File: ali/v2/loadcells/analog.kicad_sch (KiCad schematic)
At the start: 57 parts, among them J10 Conn_01x04, J11 Conn_01x04, J12 Conn_01x04, J13 Conn_01x04, J14 Conn_01x04, J9 Conn_01x04, U5 ADS124S08

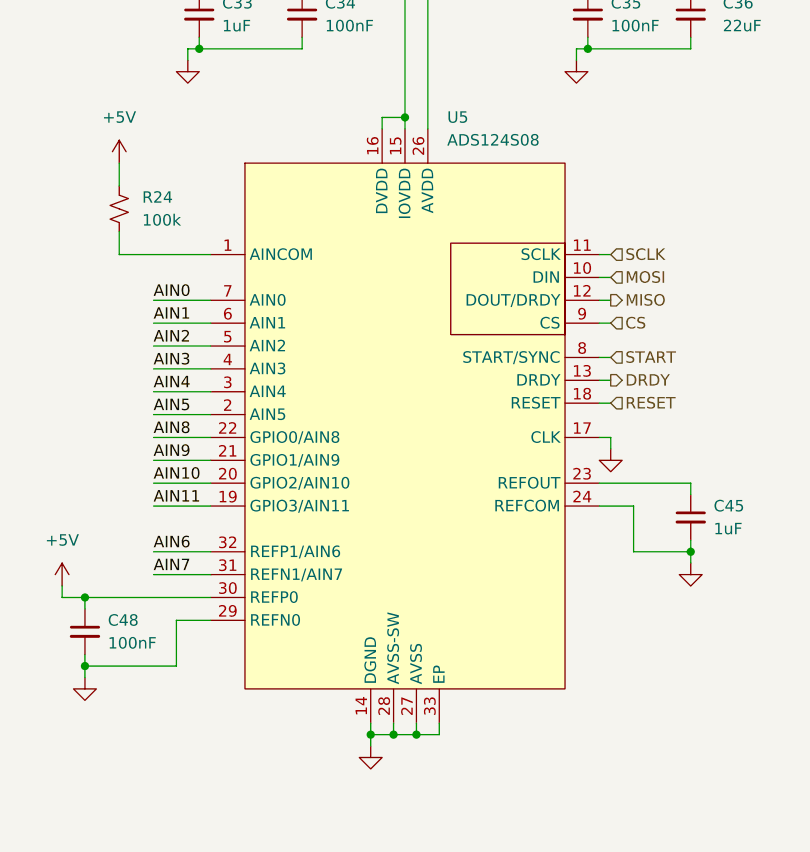
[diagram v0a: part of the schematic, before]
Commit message: mfw pts
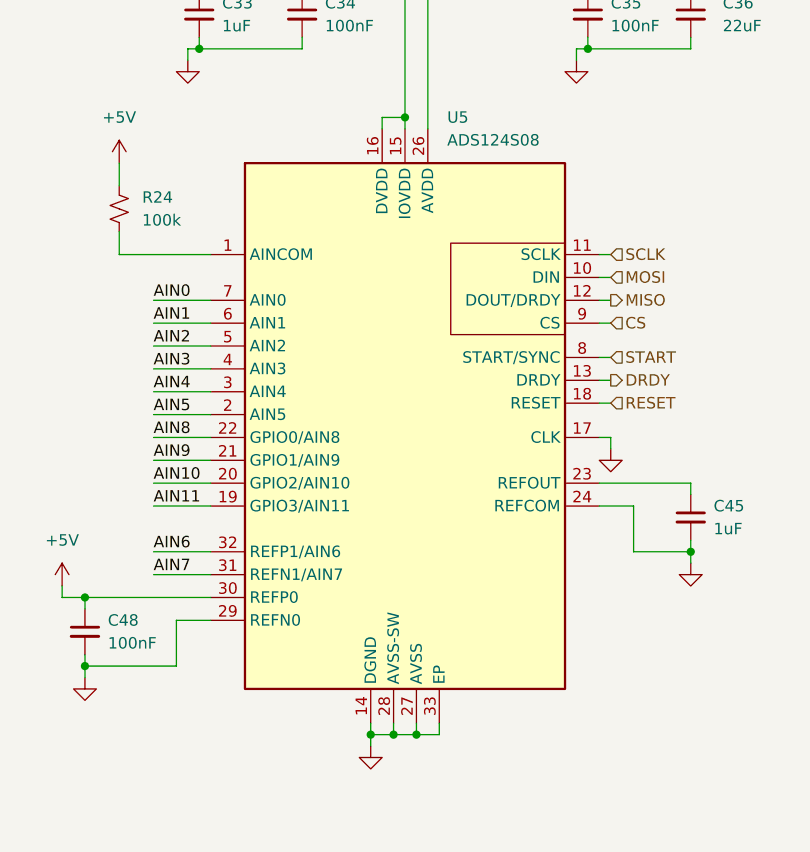
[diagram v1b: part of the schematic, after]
